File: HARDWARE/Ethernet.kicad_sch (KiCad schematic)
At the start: 27 parts, among them J4 KLS12-TL051, J5 KLS12-TL051, U7 KSZ8463FRL, U8 USBLC6-4SC6, U9 USBLC6-4SC6, Y3 25Mhz

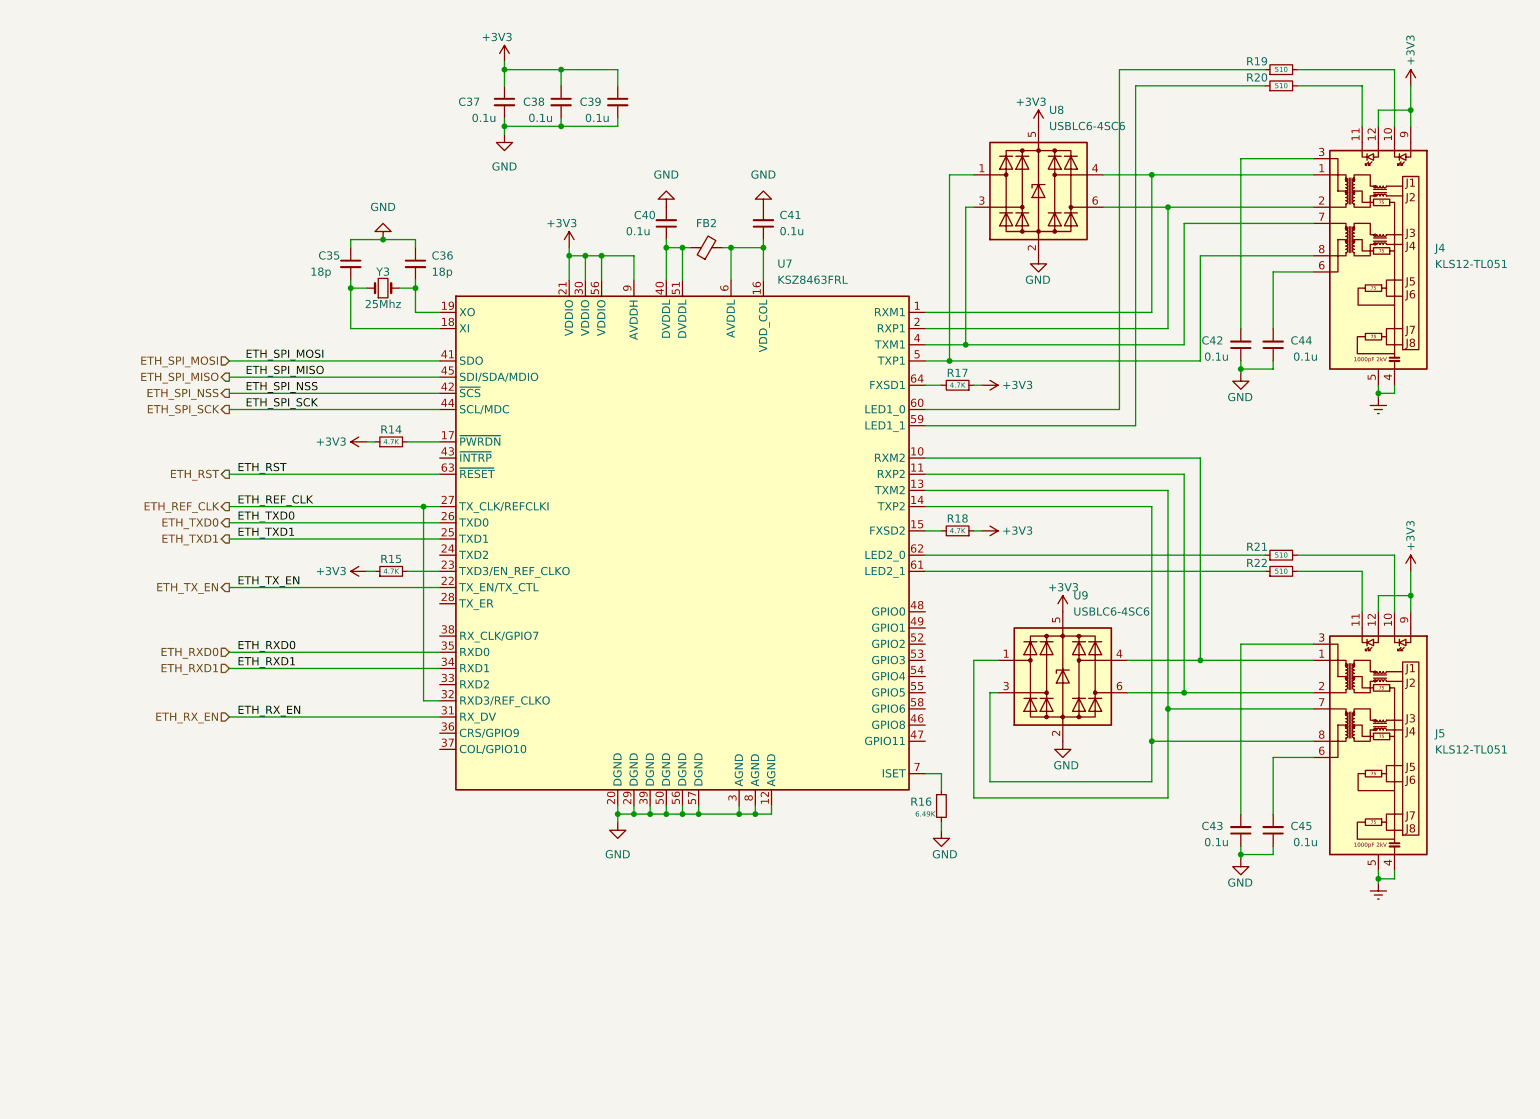
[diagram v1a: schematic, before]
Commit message: tracerouting
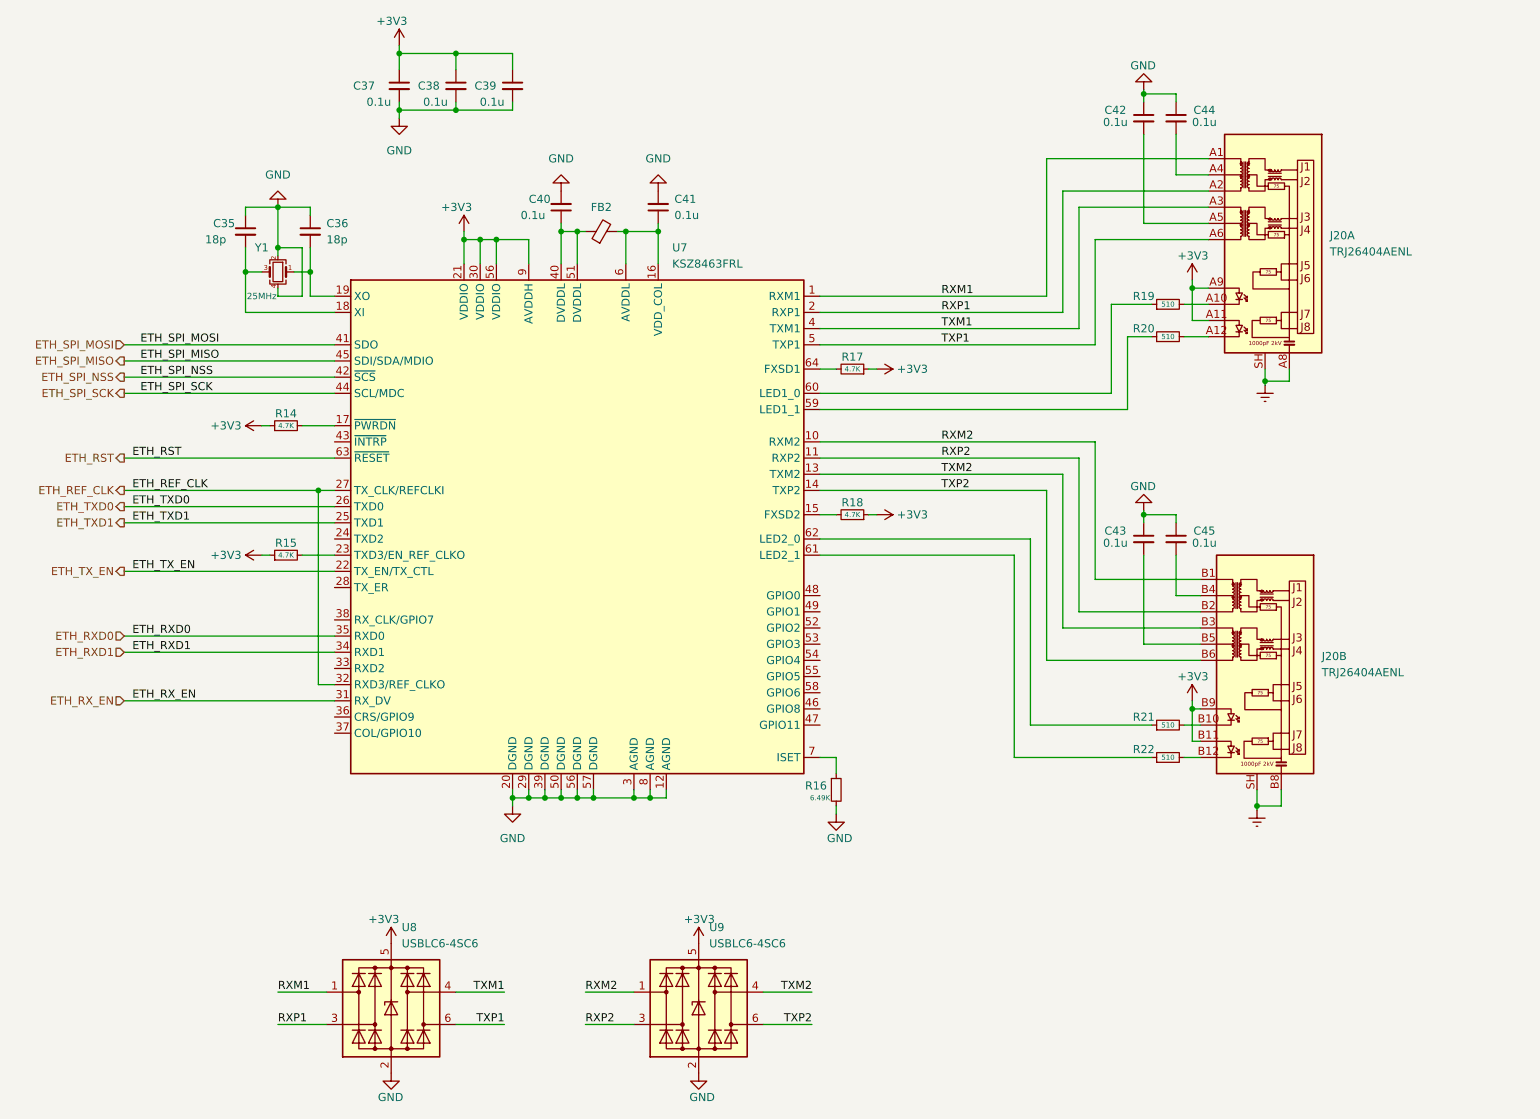
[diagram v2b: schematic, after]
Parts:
- removed J4, J5: KLS12-TL051, Footpint:KLS12-TL051, symbol meshium_duo:KLS12-TL051
- removed Y3: 25Mhz, Crystal:Crystal_SMD_3225-4Pin_3.2x2.5mm, symbol Device:Crystal_Small
- added J20: TRJ26404AENL, symbol meshium_duo:TRJ26404AENL
- added Y1: 25MHz, Crystal:Crystal_SMD_3225-4Pin_3.2x2.5mm, symbol Device:Crystal_GND24_Small
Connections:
- net +3V3: now also J20.A11 (LEDY_A), J20.A9 (LEDG_A), J20.B11 (LEDY_A), J20.B9 (LEDG_A)
- net Earth: now also J20.A8 (TERM), J20.B8 (TERM), J20.SH (SHIELD), J20.SH (SHIELD)
- net GND: now also Y1.2, Y1.4
- net at C35.2, U7.18 (XI): now also Y1.3
- net at C36.2, U7.19 (XO): now also Y1.1
- net at C45.2: now also J20.B4 (CT)
- net RXM1: now reaches U8.1 (I/O1)
- net RXM1: now also U7.1 (RXM1), J20.A1 (RD+); no longer U7.5 (TXP1)
- net RXP1: now reaches U8.3 (I/O2)
- net RXP1: now also U7.2 (RXP1), J20.A2 (RD-); no longer U7.4 (TXM1)
- net TXM1: now reaches U8.4 (I/O3)
- net TXM1: now also U7.4 (TXM1), J20.A3 (TD+); no longer U7.1 (RXM1)
- net TXP1: now reaches U8.6 (I/O4)
- net TXP1: now also U7.5 (TXP1), J20.A6 (TD-); no longer U7.2 (RXP1)
- net RXM2: now reaches U7.10 (RXM2)
- net RXM2: now also U9.1 (I/O1), J20.B1 (RD+); no longer U9.4 (I/O3)
- net RXP2: now reaches U7.11 (RXP2)
- net RXP2: now also U9.3 (I/O2), J20.B2 (RD-); no longer U9.6 (I/O4)
- net TXM2: now reaches U7.13 (TXM2)
- net TXM2: now also U9.4 (I/O3), J20.B3 (TD+); no longer U9.1 (I/O1)
- net TXP2: now reaches U7.14 (TXP2)
- net TXP2: now also U9.6 (I/O4), J20.B6 (TD-); no longer U9.3 (I/O2)
- net at R21.2: now also J20.B10 (LEDG_C)
- net at C42.2: now also J20.A5 (CT)
- net at C44.2: now also J20.A4 (CT)
- net at C43.2: now also J20.B5 (CT)
- net at R22.2: now also J20.B12 (LEDY_C)
- net at R20.2: now also J20.A12 (LEDY_C)
- net at R19.2: now also J20.A10 (LEDG_C)
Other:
- moved on the sheet: C35, C36, C37, C38, C39, C40, C41, C42, C43, C44, C45, FB2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
